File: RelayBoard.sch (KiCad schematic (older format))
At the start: 65 parts, among them P1 HE10-32, Q1 NPN, Q10 NPN, Q11 NPN, Q12 NPN, Q13 NPN, Q14 NPN, Q15 NPN, Q16 NPN, Q2 NPN, Q3 NPN, Q4 NPN, Q5 NPN, Q6 NPN, Q7 NPN, Q8 NPN, Q9 NPN

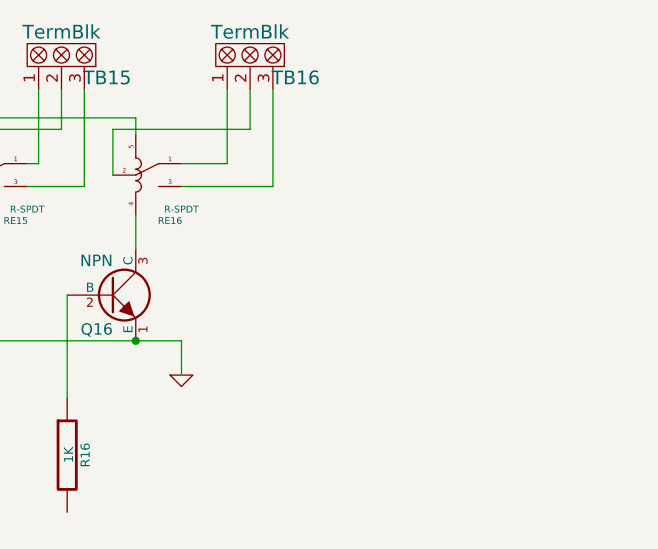
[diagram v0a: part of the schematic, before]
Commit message: End of worktime
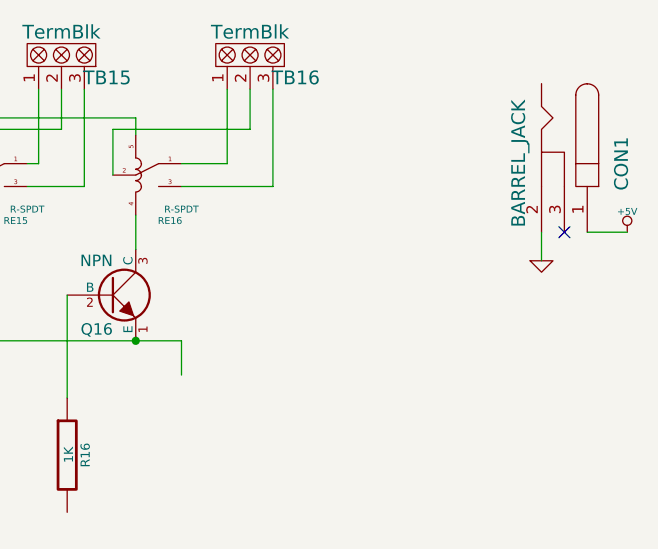
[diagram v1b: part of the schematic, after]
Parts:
- added CON1: BARREL_JACK, symbol BARREL_JACK
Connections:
- net GND: now also CON1.2; no longer Q1.1 (E), Q10.1 (E), Q11.1 (E), Q12.1 (E), Q13.1 (E), Q14.1 (E), Q15.1 (E), Q16.1 (E), Q2.1 (E), Q3.1 (E), Q4.1 (E), Q5.1 (E), Q6.1 (E), Q7.1 (E), Q8.1 (E), Q9.1 (E)
- new net: Q1.1 (E), Q10.1 (E), Q11.1 (E), Q12.1 (E), Q13.1 (E), Q14.1 (E), Q15.1 (E), Q16.1 (E), Q2.1 (E), Q3.1 (E), Q4.1 (E), Q5.1 (E), Q6.1 (E), Q7.1 (E), Q8.1 (E), Q9.1 (E)
- new net +5V: CON1.1
- no-connect marks 0 -> 1
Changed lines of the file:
@@
-$EndComp
-$Comp
-L GND #PWR01
-U 1 1 54E16FA4
-P 11250 2275
-F 0 "#PWR01" H 11250 2275 30  0001 C CNN
-F 1 "GND" H 11250 2205 30  0001 C CNN
-F 2 "" H 11250 2275 60  0000 C CNN
-F 3 "" H 11250 2275 60  0000 C CNN
-	1    11250 2275
-	1    0    0    -1
 $EndComp
 $Comp
@@
 Text GLabel 5300 2875 3    60   Input ~ 0
 Pin7
+$Comp
+L BARREL_JACK CON1
+U 1 1 54E1B203
+P 12925 1350
+F 0 "CON1" H 12925 1600 60  0000 C CNN
+F 1 "BARREL_JACK" H 12925 1150 60  0000 C CNN
+F 2 "" H 12925 1350 60  0000 C CNN
+F 3 "" H 12925 1350 60  0000 C CNN
+	1    12925 1350
+	0    1    1    0
+$EndComp
+$Comp
+L GND #PWR01
+U 1 1 54E1B226
+P 12825 1775
+F 0 "#PWR01" H 12825 1775 30  0001 C CNN
+F 1 "GND" H 12825 1705 30  0001 C CNN
+F 2 "" H 12825 1775 60  0000 C CNN
+F 3 "" H 12825 1775 60  0000 C CNN
+	1    12825 1775
+	1    0    0    -1
+$EndComp
+Wire Wire Line
+	12825 1775 12825 1650
+$Comp
+L +5V #PWR02
+U 1 1 54E1B2FB
+P 13200 1650
+F 0 "#PWR02" H 13200 1740 20  0001 C CNN
+F 1 "+5V" H 13200 1740 30  0000 C CNN
+F 2 "" H 13200 1650 60  0000 C CNN
+F 3 "" H 13200 1650 60  0000 C CNN
+	1    13200 1650
+	1    0    0    -1
+$EndComp
+Wire Wire Line
+	13025 1650 13200 1650
+NoConn ~ 12925 1650
 $EndSCHEMATC
